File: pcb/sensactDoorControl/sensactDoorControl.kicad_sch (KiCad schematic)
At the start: 54 parts, among them J1 Finger_large, J10 Fingerprint, J11 G19, J12 G23, J13 I2C, J2 Can+24V, J3 RS485, J4 PROG, J5 Motor, J8 G4_PU, J9 G16, Q1 BC847, SW1 Boot, SW2 Reset, SW3 ON TERM, SW4 TERM ON, U1 ESP32-WROOM-E, U2 TPS54202DDC, U3 PC817, U4 SN65HVD230, U5 MAX3485

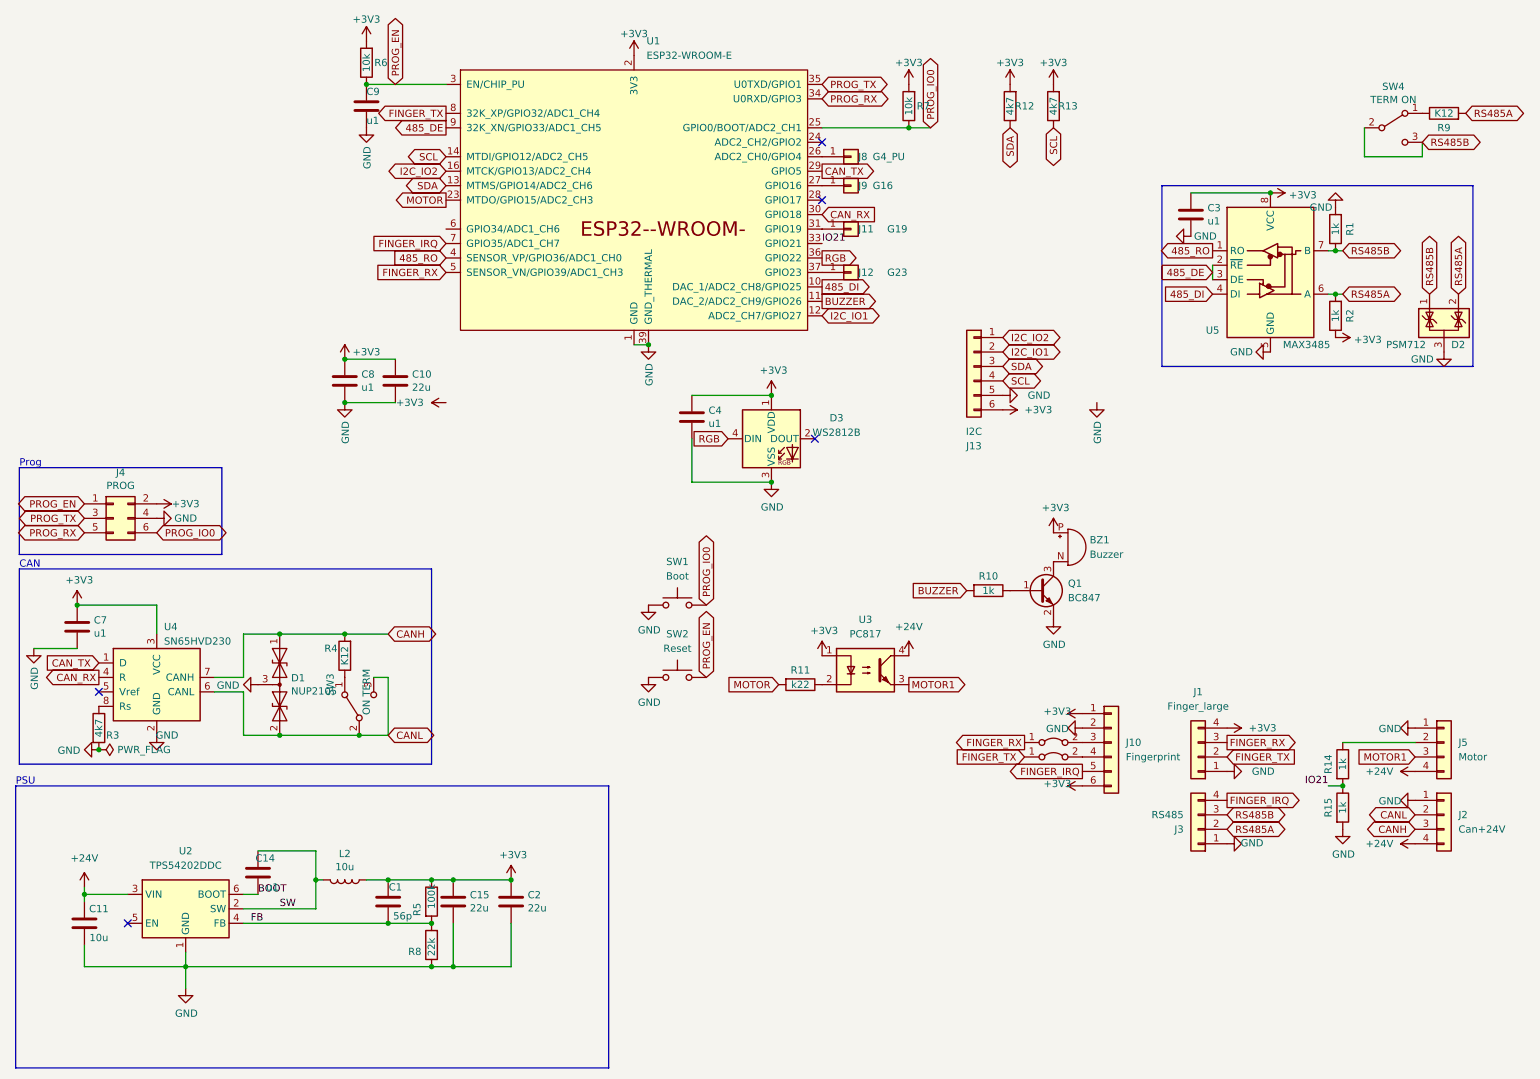
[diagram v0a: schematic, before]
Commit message: DorrControl PCB improved 2.0
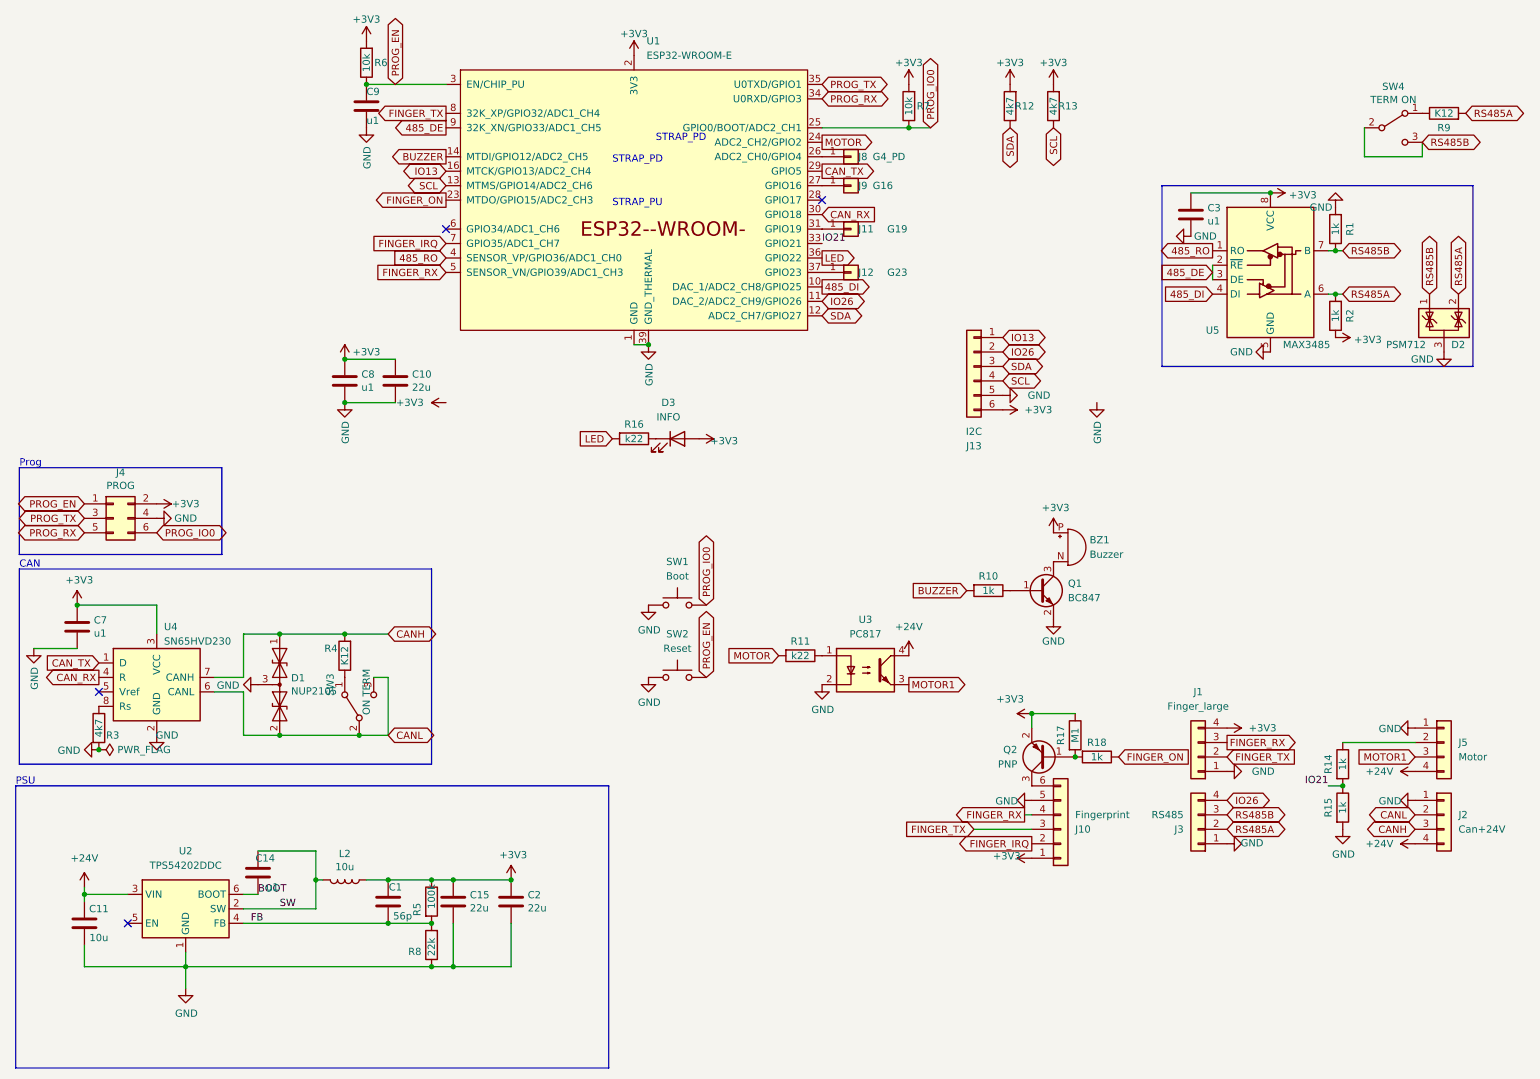
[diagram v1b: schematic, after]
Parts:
- removed C4: u1, Capacitor_SMD:C_0805_2012Metric_Pad1.18x1.45mm_HandSolder, symbol Device:C
- removed D3: WS2812B, liebler_OPTO:WS2812b_handsolder, symbol LED:WS2812B
- removed JP1: RX, Jumper:SolderJumper-2_P1.3mm_Bridged_RoundedPad1.0x1.5mm, symbol Jumper:Jumper_2_Bridged
- removed JP2: TX, Jumper:SolderJumper-2_P1.3mm_Bridged_RoundedPad1.0x1.5mm, symbol Jumper:Jumper_2_Bridged
- added D3: INFO, LED_SMD:LED_0805_2012Metric_Pad1.15x1.40mm_HandSolder, symbol Device:LED
- added Q2: PNP, Package_TO_SOT_SMD:SOT-23_Handsoldering, symbol Transistor_BJT:BC857
- added R16: k22, Resistor_SMD:R_0805_2012Metric_Pad1.20x1.40mm_HandSolder, symbol Device:R
- added R17: M1, Resistor_SMD:R_0805_2012Metric_Pad1.20x1.40mm_HandSolder, symbol Device:R
- added R18: 1k, Resistor_SMD:R_0805_2012Metric_Pad1.20x1.40mm_HandSolder, symbol Device:R
- J8: value G4_PU -> G4_PD
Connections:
- net +3V3: now also D3.2 (A), Q2.2 (E), R17.1; no longer J10.6 (Pin_6), U3.1
- net BUZZER: now also U1.14 (MTDI/GPIO12/ADC2_CH5); no longer U1.11 (DAC_2/ADC2_CH9/GPIO26)
- net FINGER_IRQ: now also J10.2 (Pin_2); no longer J10.5 (Pin_5), J3.4 (Pin_4)
- net FINGER_RX: now also J10.4 (Pin_4)
- net FINGER_TX: now also J10.3 (Pin_3)
- net GND: now also J10.5 (Pin_5), SW2.2, U3.2; no longer J10.2 (Pin_2), SW2.1
- net MOTOR: now also U1.24 (ADC2_CH2/GPIO2); no longer U1.23 (MTDO/GPIO15/ADC2_CH3)
- net PROG_EN: now also SW2.1; no longer SW2.2
- net SCL: now also U1.13 (MTMS/GPIO14/ADC2_CH6); no longer U1.14 (MTDI/GPIO12/ADC2_CH5)
- net SDA: now also U1.12 (ADC2_CH7/GPIO27); no longer U1.13 (MTMS/GPIO14/ADC2_CH6)
- net at R11.1: now also U3.1; no longer U3.2
- net I2C_IO1 renamed IO26
- net IO26: now also J3.4 (Pin_4), U1.11 (DAC_2/ADC2_CH9/GPIO26); no longer U1.12 (ADC2_CH7/GPIO27)
- net I2C_IO2 renamed IO13
- net RGB renamed LED
- net LED: now also R16.2
- new net: J10.6 (Pin_6), Q2.3 (C)
- new net: D3.1 (K), R16.1
- new net: Q2.1 (B), R17.2, R18.2
- new net FINGER_ON: R18.1, U1.23 (MTDO/GPIO15/ADC2_CH3)
- no-connect marks 5 -> 4
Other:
- note added: "STRAP_PD"
- note added: "STRAP_PU"
- moved on the sheet: J10, R11

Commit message: sensactDoorControl as sent to JLCPCB
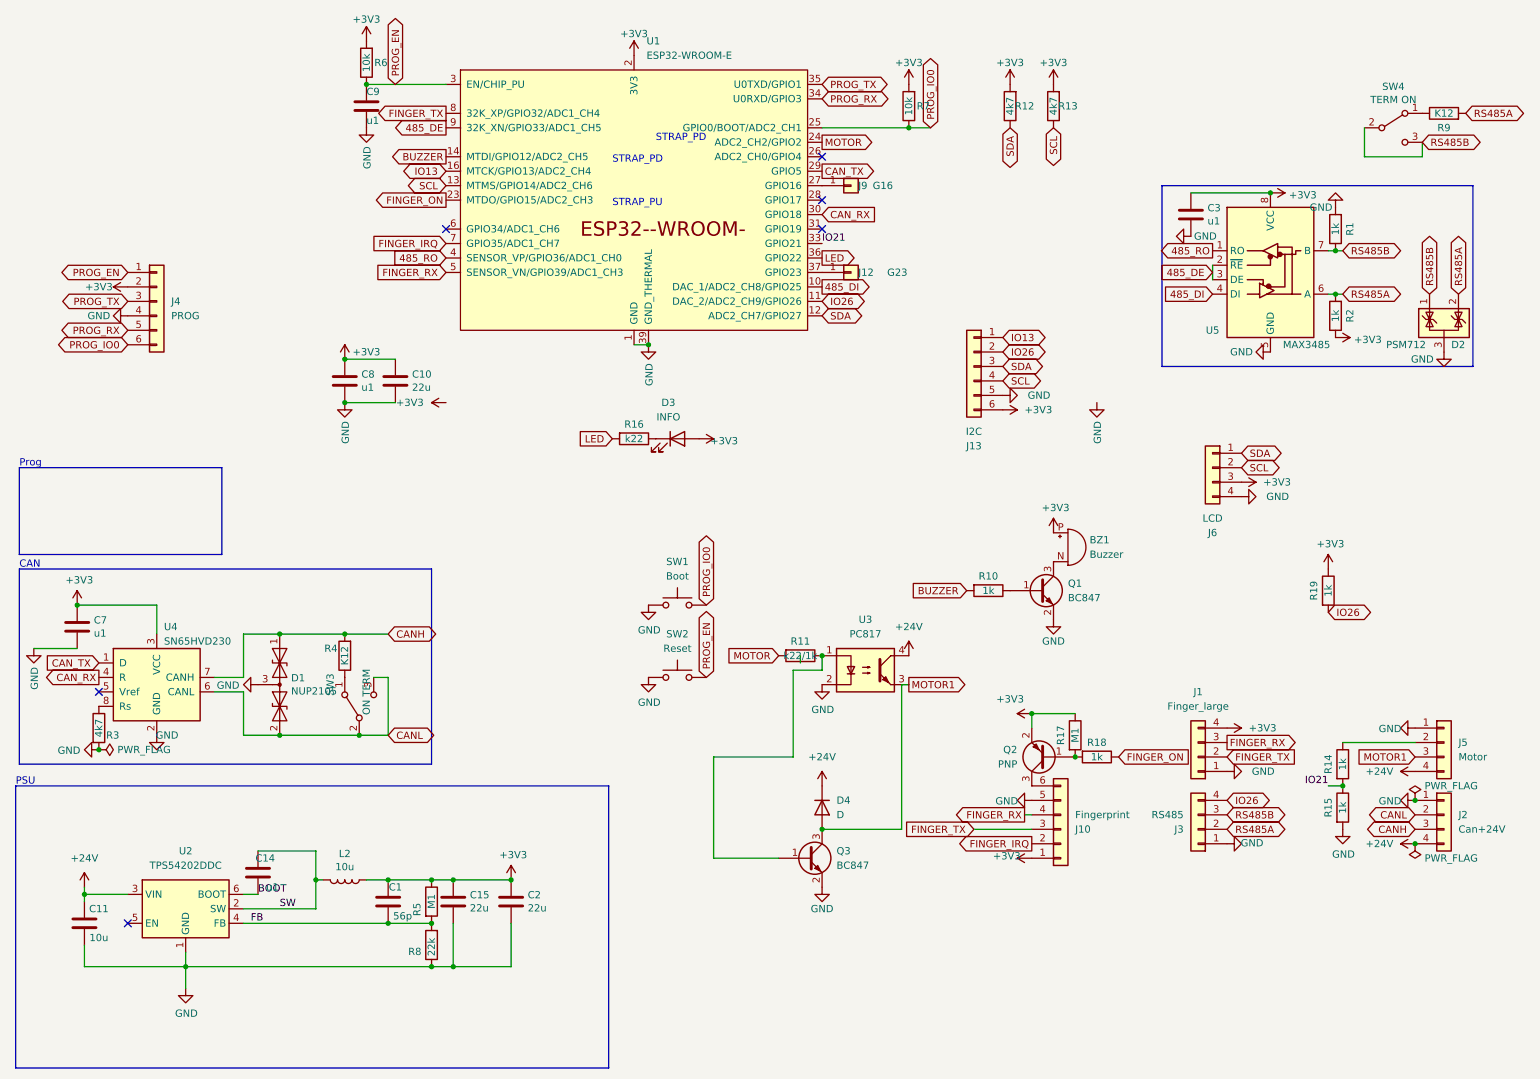
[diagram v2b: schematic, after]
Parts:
- removed J11: G19, TestPoint:TestPoint_THTPad_D1.5mm_Drill0.7mm, symbol Connector_Generic:Conn_01x01
- removed J4: PROG, liebler_CONN:IDC_2x03_P1.27mm_Vertical, symbol Connector_Generic:Conn_02x03_Odd_Even
- removed J8: G4_PD, TestPoint:TestPoint_THTPad_D1.5mm_Drill0.7mm, symbol Connector_Generic:Conn_01x01
- added D4: D, liebler_SEMICONDUCTORS:D_SOD-123_handsolder, symbol Device:D
- added J4: PROG, liebler_CONN:JST_SH_SM06B-SRSS-TB_1x06-1MP_P1.00mm_Horizontal_handsolder, symbol Connector_Generic:Conn_01x06
- added J6: LCD, Connector_PinHeader_2.54mm:PinHeader_1x04_P2.54mm_Vertical, symbol Connector_Generic:Conn_01x04
- added Q3: BC847, Package_TO_SOT_SMD:SOT-23_Handsoldering, symbol Transistor_BJT:BC847
- added R19: 1k, Resistor_SMD:R_0805_2012Metric_Pad1.20x1.40mm_HandSolder, symbol Device:R
- R11: value k22 -> k22/1k
- R5: value 100k -> M1
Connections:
- net +24V: now also D4.1 (K)
- net +3V3: now also J4.2 (Pin_2), J6.3 (Pin_3), R19.1
- net GND: now also J4.4 (Pin_4), J6.4 (Pin_4), Q3.2 (E)
- net IO26: now also R19.2
- net MOTOR1: now also D4.2 (A), Q3.3 (C)
- net PROG_EN: now also J4.1 (Pin_1)
- net PROG_IO0: now also J4.6 (Pin_6)
- net PROG_RX: now also J4.5 (Pin_5)
- net PROG_TX: now also J4.3 (Pin_3)
- net SCL: now also J6.2 (Pin_2)
- net SDA: now also J6.1 (Pin_1)
- net at R11.1, U3.1: now also Q3.1 (B)
- no-connect marks 4 -> 6

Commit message: Minor Changes
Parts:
- J6: footprint Connector_PinHeader_2.54mm:PinHeader_1x04_P2.54mm_Vertical -> Connector_PinSocket_2.54mm:PinSocket_1x04_P2.54mm_Vertical
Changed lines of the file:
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@@
       (effects (font (size 1.27 1.27)))
     )
-    (property "Footprint" "Connector_PinHeader_2.54mm:PinHeader_1x04_P2.54mm_Vertical" (at 228.6 90.17 0)
+    (property "Footprint" "Connector_PinSocket_2.54mm:PinSocket_1x04_P2.54mm_Vertical" (at 228.6 90.17 0)
       (effects (font (size 1.27 1.27)) hide)
     )
